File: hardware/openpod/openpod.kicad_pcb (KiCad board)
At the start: 2 copper layers, 65 x 95.3 mm, 20 parts, among them U1 STM32F446RCTx

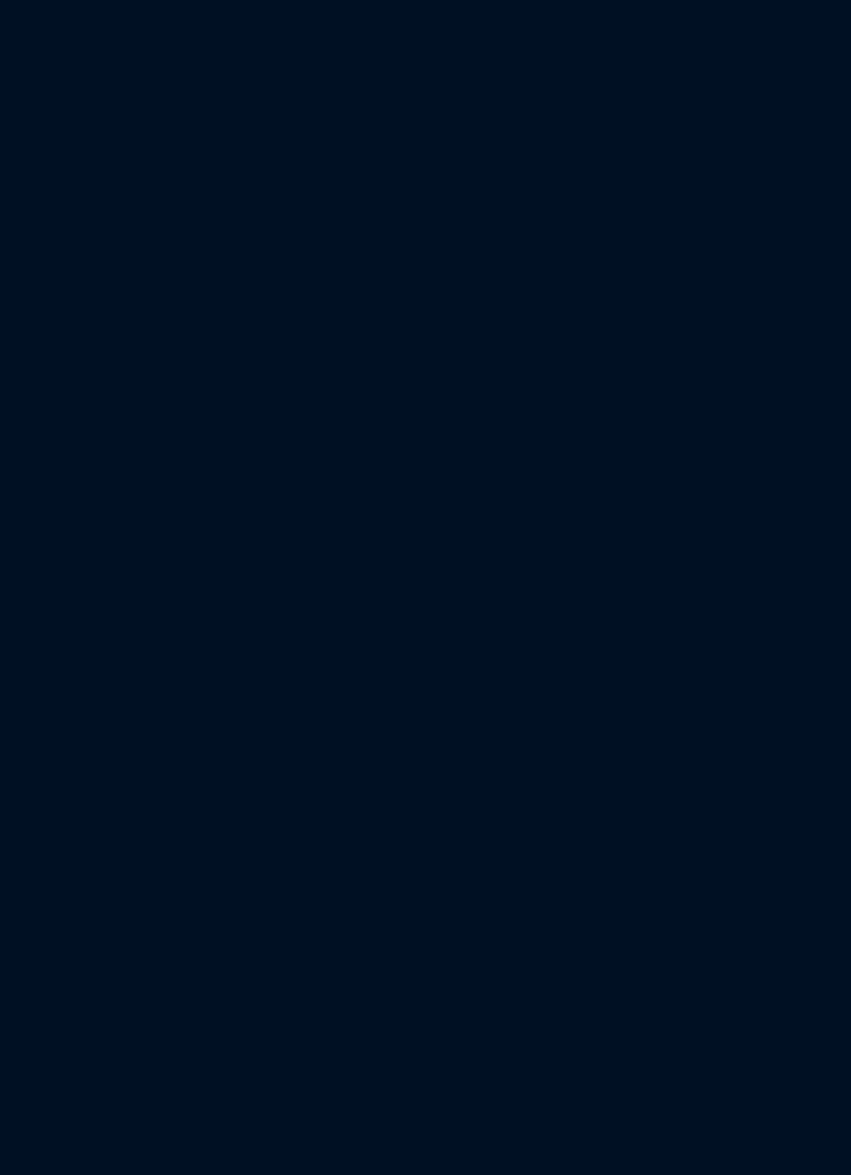
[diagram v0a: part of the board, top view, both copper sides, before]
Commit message: dev boards
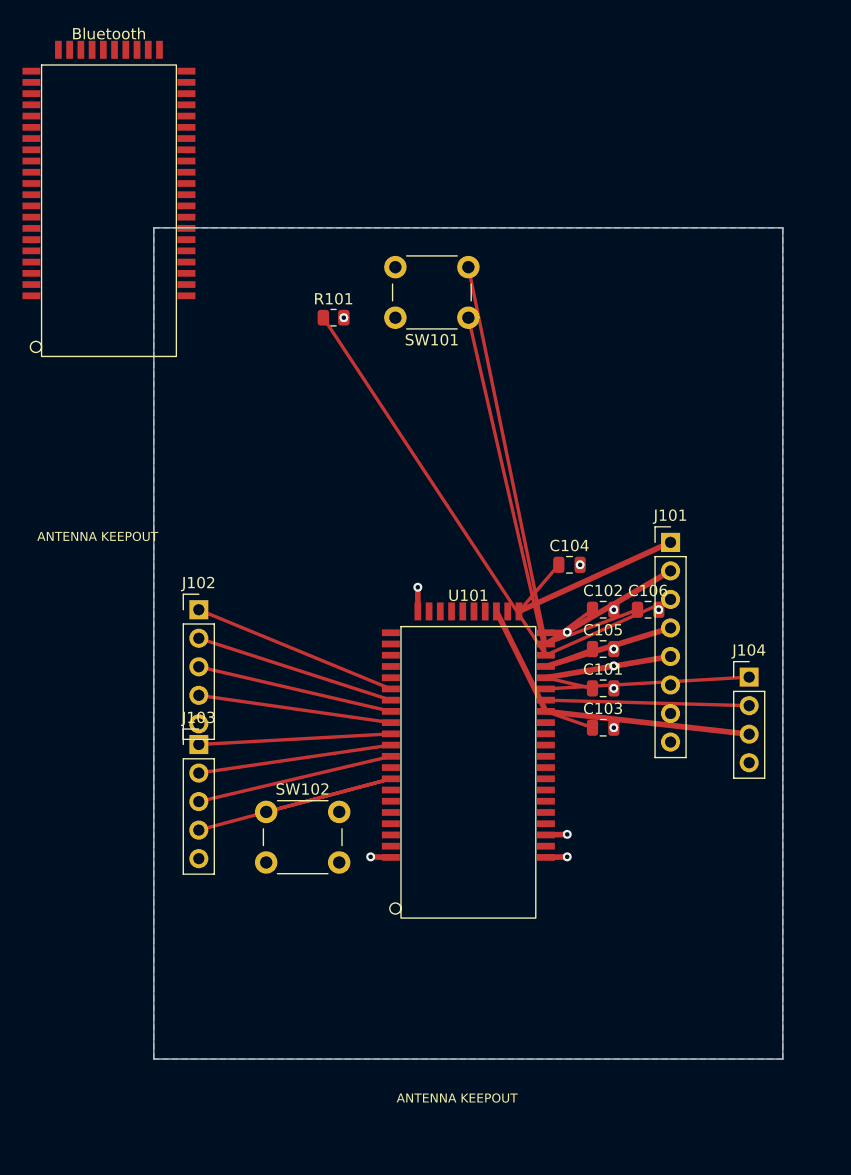
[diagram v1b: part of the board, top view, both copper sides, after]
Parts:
- added Bluetooth: ~, openpod:fsc-bt1035, F.Cu at (0.00, 0.00)
- added C101: 100n, Capacitor_SMD:C_0805_2012Metric, F.Cu at (44.0, 43.0)
- added C102: 100n, Capacitor_SMD:C_0805_2012Metric, F.Cu at (44.0, 36.0)
- added C103: 100n, Capacitor_SMD:C_0805_2012Metric, F.Cu at (44.0, 46.5)
- added C104: 100n, Capacitor_SMD:C_0805_2012Metric, F.Cu at (41.0, 32.0)
- added C105: 100n, Capacitor_SMD:C_0805_2012Metric, F.Cu at (44.0, 39.5)
- added C106: 10u, Capacitor_SMD:C_0805_2012Metric, F.Cu at (48.0, 36.0)
- added J101: POWER, Connector_PinHeader_2.54mm:PinHeader_1x08_P2.54mm_Vertical, F.Cu at (50.0, 30.0)
- added J102: UART, Connector_PinHeader_2.54mm:PinHeader_1x05_P2.54mm_Vertical, F.Cu at (8.00, 36.0)
- added J103: DEBUG, Connector_PinHeader_2.54mm:PinHeader_1x05_P2.54mm_Vertical, F.Cu at (8.00, 48.0)
- added J104: USB, Connector_PinHeader_2.54mm:PinHeader_1x04_P2.54mm_Vertical, F.Cu at (57.0, 42.0)
- added R101: 100k, Resistor_SMD:R_0805_2012Metric, F.Cu at (20.0, 10.0)
- added SW101: PWR, Button_Switch_THT:SW_PUSH_6mm_H4.3mm, F.Cu at (32.0, 10.0)
- added SW102: RST, Button_Switch_THT:SW_PUSH_6mm_H4.3mm, F.Cu at (14.0, 54.0)
- added U101: FSC-BT1035, openpod:fsc-bt1035, F.Cu at (32.0, 50.0)
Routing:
- net BT_SYS_CTRL: track 0.00 -> 79.0 mm
- net BT_VBAT: track 0.00 -> 61.0 mm
- net BT_VCHG: track 0.00 -> 32.5 mm
- net BT_RESET: track 0.00 -> 29.2 mm
- net BT_3V3: track 0.00 -> 20.3 mm
- net BT_RTS: track 0.00 -> 18.5 mm
- net BT_USB_DP: track 0.00 -> 18.1 mm
- net BT_USB_DN: track 0.00 -> 18.1 mm
- net BT_CTS: track 0.00 -> 18.0 mm
- net BT_PIO6: track 0.00 -> 17.6 mm
- net BT_RX: track 0.00 -> 17.6 mm
- net BT_PIO7: track 0.00 -> 17.3 mm
- net BT_TX: track 0.00 -> 17.3 mm
- net BT_PIO8: track 0.00 -> 17.1 mm
- net BT_1V8: track 0.00 -> 16.0 mm
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- added copper zone on B.Cu, net BT_GND
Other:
- board size 65 x 95.3 mm -> 161.1 x 143.3 mm
